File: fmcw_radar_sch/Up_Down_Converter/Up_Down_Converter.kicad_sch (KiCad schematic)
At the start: 9 parts, among them J1 Conn_01x04_Pin, J10 Screw_Terminal_01x05, J2 Conn_01x04_Pin, J3 Conn_Coaxial, J4 Conn_01x04_Pin

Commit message: layout
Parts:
- J3: footprint (none) -> Connector_Coaxial:SMA_Amphenol_132134-10_Vertical
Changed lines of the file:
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@@
 			)
 		)
-		(property "Footprint" ""
+		(property "Footprint" "Connector_Coaxial:SMA_Amphenol_132134-10_Vertical"
 			(at 181.61 121.92 0)
 			(effects

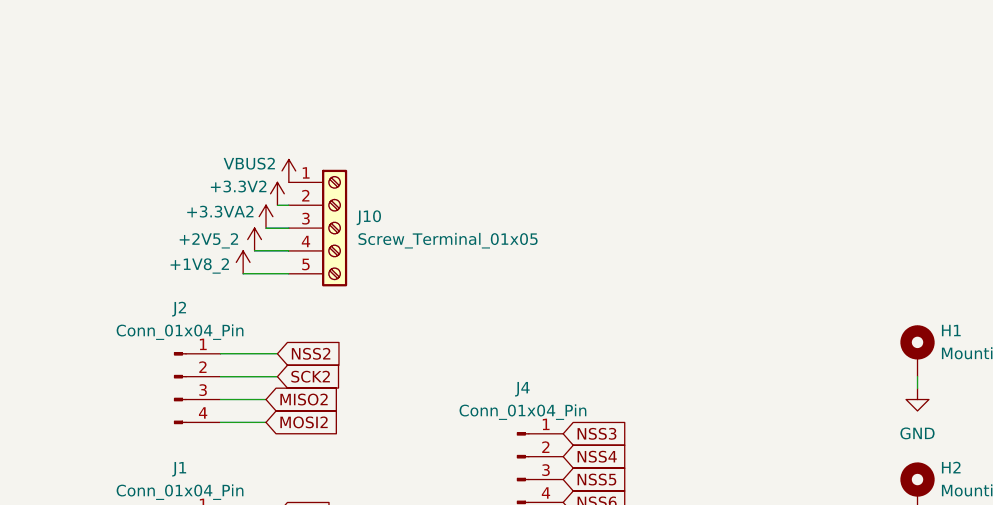
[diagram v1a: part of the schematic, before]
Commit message: a lot of updates
usb power delivery + finishing touches
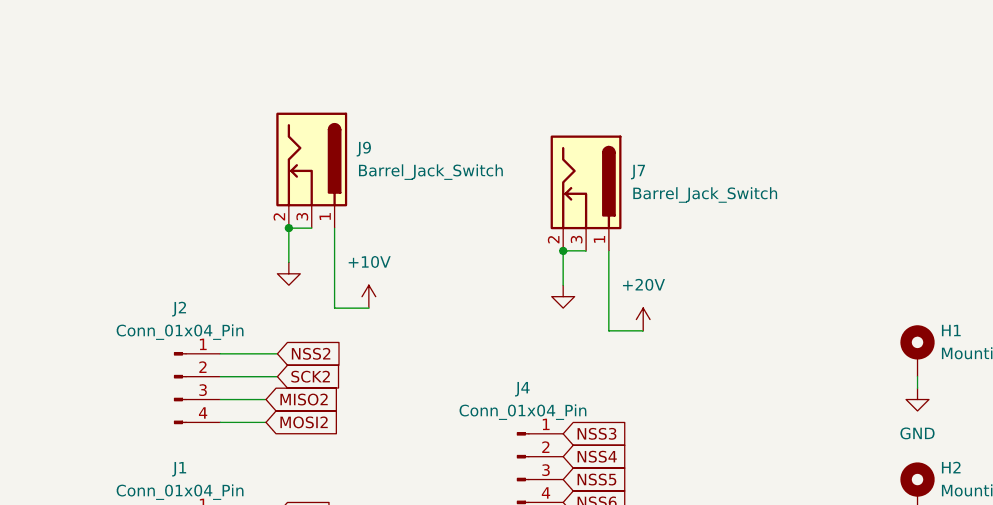
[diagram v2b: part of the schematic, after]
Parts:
- removed J10: Screw_Terminal_01x05, TerminalBlock_Phoenix:TerminalBlock_Phoenix_MKDS-3-5-5.08_1x05_P5.08mm_Horizontal, symbol Connector:Screw_Terminal_01x05
- added J7, J9: Barrel_Jack_Switch, symbol Connector:Barrel_Jack_Switch
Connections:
- net GND: now also J7.2, J7.3, J9.2, J9.3
- new net +10V: J9.1
- new net +20V: J7.1

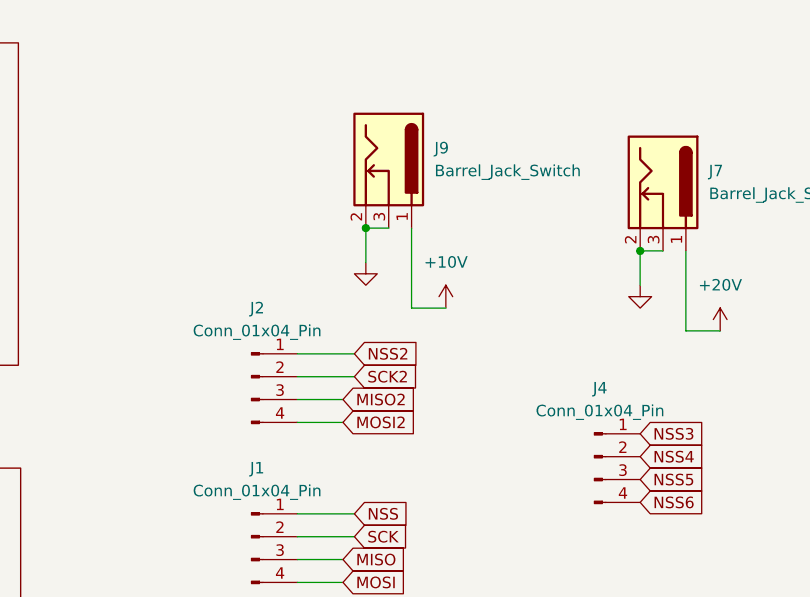
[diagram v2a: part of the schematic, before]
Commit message: Silkscreen finishing
Silkscreen finishting
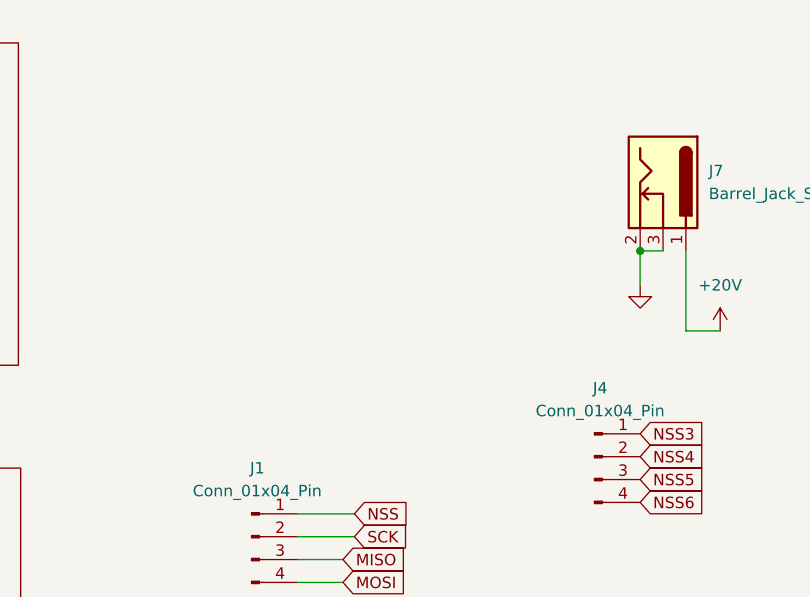
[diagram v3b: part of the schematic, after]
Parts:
- removed J2: Conn_01x04_Pin, Connector_PinHeader_2.54mm:PinHeader_1x04_P2.54mm_Vertical, symbol Connector:Conn_01x04_Pin
- removed J9: Barrel_Jack_Switch, symbol Connector:Barrel_Jack_Switch
- J7: footprint (none) -> Connector_BarrelJack:BarrelJack_Horizontal
